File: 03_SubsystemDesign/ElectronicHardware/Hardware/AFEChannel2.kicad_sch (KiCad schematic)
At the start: 30 parts, among them U2101 OPA690xDBV, U2102 AD8139

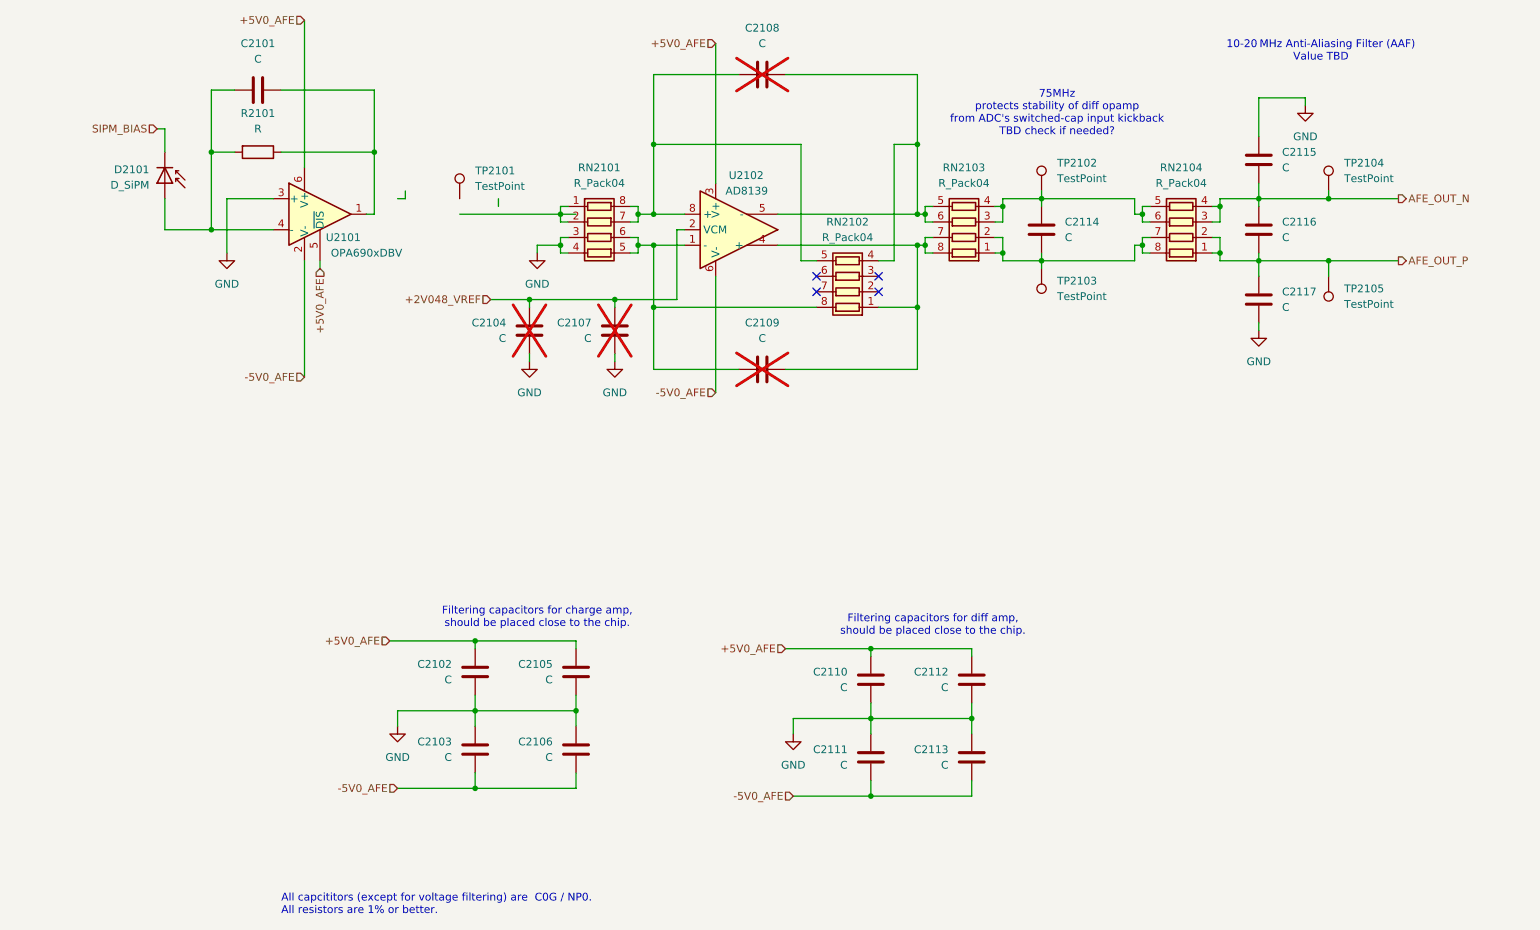
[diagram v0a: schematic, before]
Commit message: pcb design work in progress
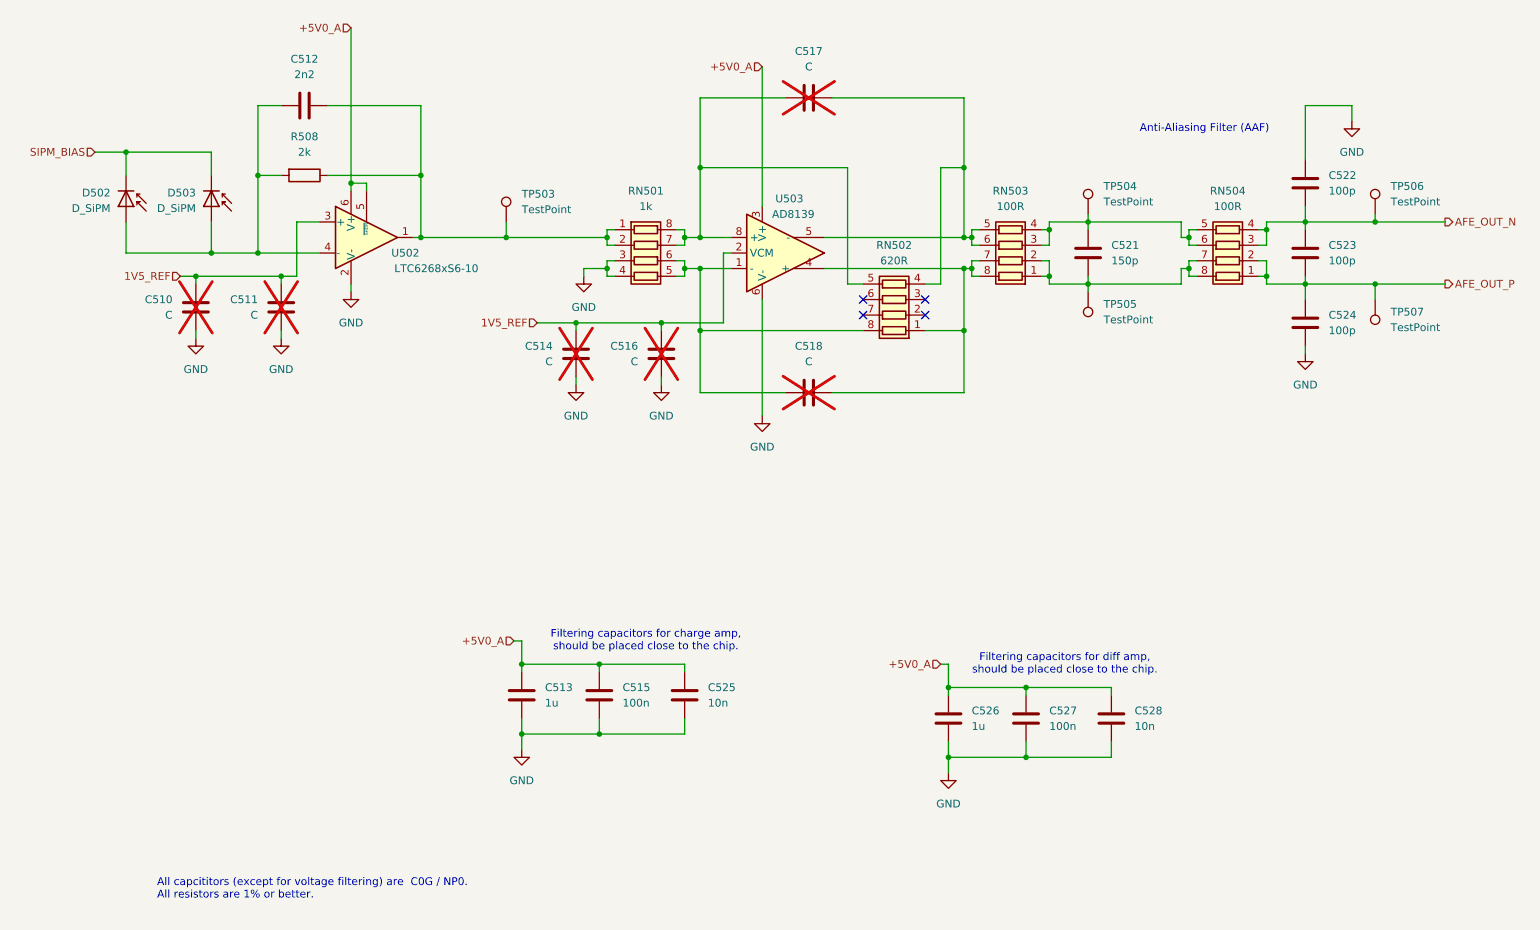
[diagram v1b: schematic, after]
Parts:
- removed C2101, C2102, C2103, C2104, C2105, C2106, C2107, C2108, C2109, C2110, C2111, C2112, C2113, C2114, C2115, C2116, C2117: C, Capacitor_SMD:C_0805_2012Metric, symbol Device:C
- removed D2101: D_SiPM, symbol Device:D_SiPM
- removed R2101: R, Resistor_SMD:R_0805_2012Metric, symbol Device:R
- removed RN2101, RN2102, RN2103, RN2104: R_Pack04, Resistor_SMD:R_Array_Convex_4x0612, symbol Device:R_Pack04
- removed TP2101, TP2102, TP2103, TP2104, TP2105: TestPoint, TestPoint:TestPoint_Pad_D1.0mm, symbol Connector:TestPoint
- removed U2101: OPA690xDBV, Package_TO_SOT_SMD:SOT-23-6, symbol Amplifier_Operational:OPA690xDBV
- removed U2102: AD8139, Package_SO:SOIC-8_5.3x5.3mm_P1.27mm, symbol GammaSpectrometer:AD8139
- added C510, C511, C514, C516, C517, C518: C, Capacitor_SMD:C_0805_2012Metric, symbol Device:C
- added C512: 2n2, Capacitor_SMD:C_0805_2012Metric, symbol Device:C
- added C513, C526: 1u, Capacitor_SMD:C_0805_2012Metric, symbol Device:C
- added C515, C527: 100n, Capacitor_SMD:C_0805_2012Metric, symbol Device:C
- added C521: 150p, Capacitor_SMD:C_0805_2012Metric, symbol Device:C
- added C522, C523, C524: 100p, Capacitor_SMD:C_0805_2012Metric, symbol Device:C
- added C525, C528: 10n, Capacitor_SMD:C_0805_2012Metric, symbol Device:C
- added D502, D503: D_SiPM, symbol Device:D_SiPM
- added R508: 2k, Resistor_SMD:R_0805_2012Metric, symbol Device:R
- added RN501: 1k, Resistor_SMD:R_Array_Convex_4x0612, symbol Device:R_Pack04
- added RN502: 620R, Resistor_SMD:R_Array_Convex_4x0612, symbol Device:R_Pack04
- added RN503, RN504: 100R, Resistor_SMD:R_Array_Convex_4x0612, symbol Device:R_Pack04
- added TP503, TP504, TP505, TP506, TP507: TestPoint, TestPoint:TestPoint_Pad_D1.0mm, symbol Connector:TestPoint
- added U502: LTC6268xS6-10, Package_TO_SOT_SMD:TSOT-23-6, symbol Amplifier_Operational:LTC6268xS6-10
- added U503: AD8139, Package_SO:SOIC-8_5.3x5.3mm_P1.27mm, symbol GammaSpectrometer:AD8139
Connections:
- net AFE_OUT_N: now also C522.1, C523.2, RN504.3 (R3.1), RN504.4 (R4.1), TP506.1
- net AFE_OUT_P: now also C523.1, C524.2, RN504.1 (R1.1), RN504.2 (R2.1), TP507.1
- net GND: now also C510.2, C511.2, C513.2, C514.2, C515.2, C516.2, C522.2, C524.1, C525.2, C526.2, C527.2, C528.2, RN501.3 (R3.1), RN501.4 (R4.1), U502.2 (V-), U503.6 (V-)
- net SIPM_BIAS: now also D502.1 (K), D503.1 (K)
- new net: C521.1, RN503.1 (R1.1), RN503.2 (R2.1), RN504.7 (R2.2), RN504.8 (R1.2), TP505.1
- new net: C521.2, RN503.3 (R3.1), RN503.4 (R4.1), RN504.5 (R4.2), RN504.6 (R3.2), TP504.1
- new net: C517.2, RN502.4 (R4.1), RN503.5 (R4.2), RN503.6 (R3.2), U503.5 (-)
- new net: C518.2, RN502.1 (R1.1), RN503.7 (R2.2), RN503.8 (R1.2), U503.4 (+)
- new net: C512.2, R508.1, RN501.1 (R1.1), RN501.2 (R2.1), TP503.1, U502.1
- new net: C512.1, D502.2 (A), D503.2 (A), R508.2, U502.4 (-)
- new net: C518.1, RN501.5 (R4.2), RN501.6 (R3.2), RN502.8 (R1.2), U503.1 (-)
- new net: C517.1, RN501.7 (R2.2), RN501.8 (R1.2), RN502.5 (R4.2), U503.8 (+)
- new net +5V0_A: C513.1, C515.1, C525.1, C526.1, C527.1, C528.1, U502.5 (~{SHDN}), U502.6 (V+), U503.3 (V+)
- new net 1V5_REF: C510.1, C511.1, C514.1, C516.1, U502.3 (+), U503.2 (VCM)
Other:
- note added: "Anti-Aliasing Filter (AAF)"
- note removed: "10-20 MHz Anti-Aliasing Filter (AAF) Value TBD"
- note removed: "75MHz protects stability of diff opamp from ADC's switched-cap input kickback TBD check if needed?"
